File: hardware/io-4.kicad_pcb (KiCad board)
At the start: 2 copper layers, 35 x 35 mm, 28 parts, among them J1 AKL_5_2, J2 AKL_5_2, J3 AKL_5_2, J4 AKL_5_2, J5 AKL_5_2, P1 CON-SENSOR2, P2 DEBUG, P3 BOOT, U1 XMC1XXX24, U2 DRILL, U3 DRILL, U4 DRILL, U5 DRILL

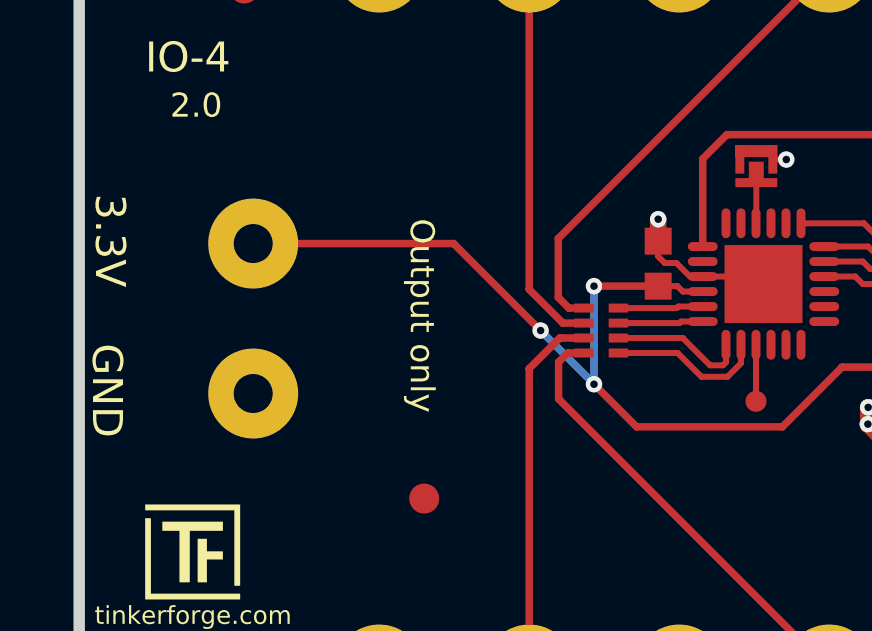
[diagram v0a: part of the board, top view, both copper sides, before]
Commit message: change description text
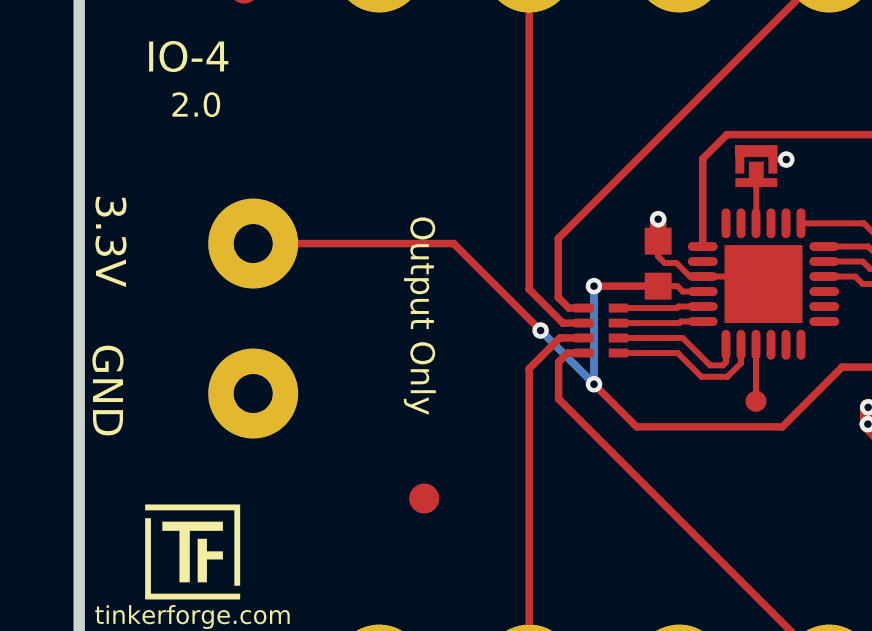
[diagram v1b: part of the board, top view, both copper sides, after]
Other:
- board text added: "Output Only"
- board text removed: "Output only"
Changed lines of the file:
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@@
     (effects (font (size 1.00076 1.00076) (thickness 0.14986)))
   )
-  (gr_text "Output only" (at 135.12302 84.3026 270) (layer F.SilkS)
+  (gr_text "Output Only" (at 135.12302 84.3026 270) (layer F.SilkS)
     (effects (font (size 0.8001 0.8001) (thickness 0.14986)))
   )
